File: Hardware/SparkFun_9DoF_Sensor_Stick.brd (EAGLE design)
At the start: 34.3 x 10.2 mm, 32 parts, among them U1 ITG-32001:1, U2 ADXL345", U3 3.3V/150mA, U4 HMC5883LSMD

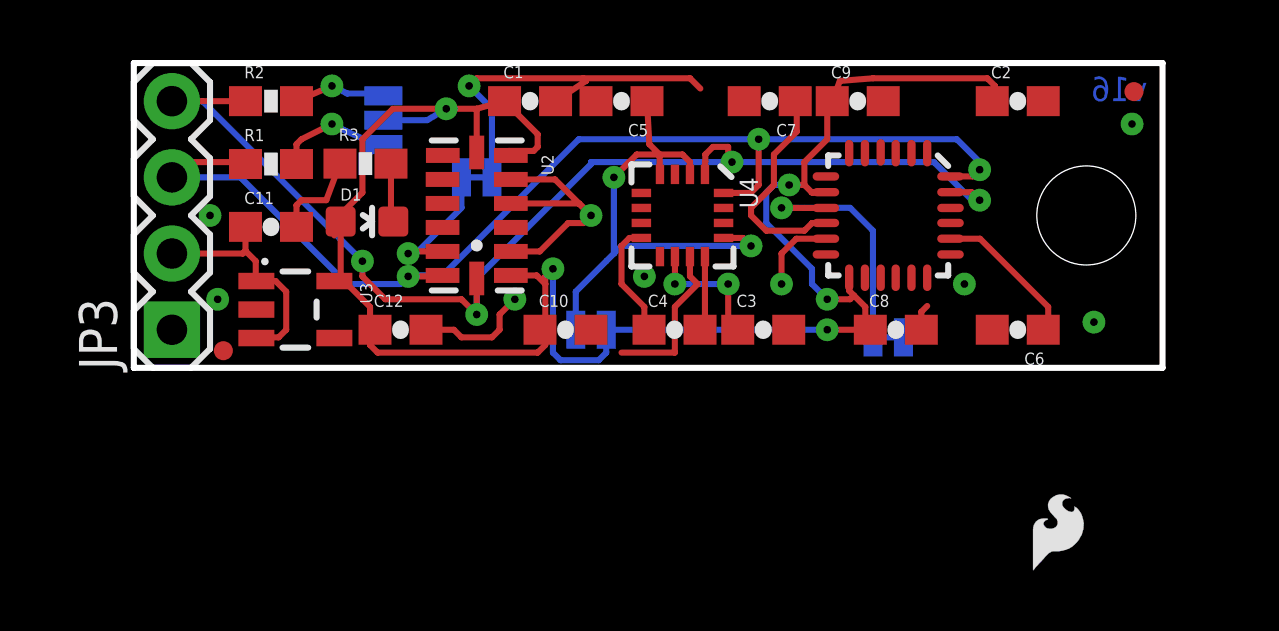
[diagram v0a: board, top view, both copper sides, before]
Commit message: BOARD PROTO LAYOUT
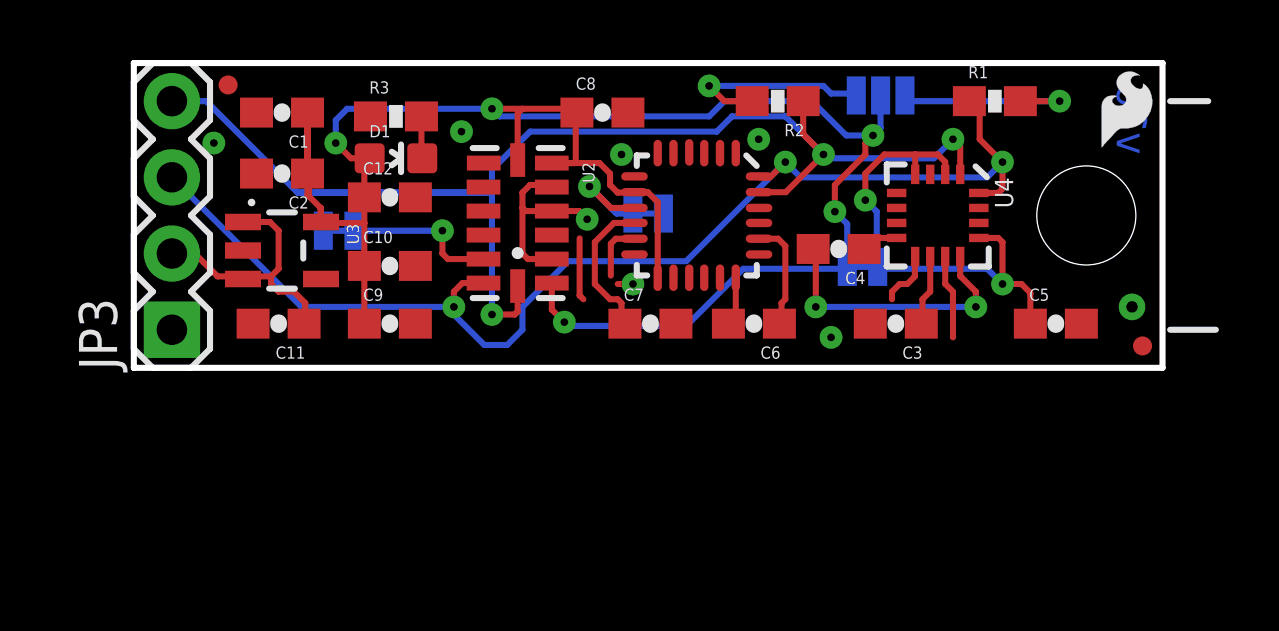
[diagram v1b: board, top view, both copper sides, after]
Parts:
- moved JP2 30.6 mm to (33.6, 0.73)
- moved JP1 30.2 mm to (3.14, 9.43)
- moved U$3 27.7 mm to (8.48, 1.75)
- moved C2 24.6 mm to (4.94, 6.48), turned to 180 degrees
- moved R1 24.2 mm to (28.7, 8.89)
- moved C9 17.3 mm to (8.53, 1.47)
- moved R2 16.9 mm to (21.5, 8.89), turned to 180 degrees
- moved SJ1 16.6 mm to (24.9, 9.08), turned to 180 degrees
- moved C5 16.3 mm to (30.7, 1.47), turned to 0 degrees
- moved JP4 14.3 mm to (31.9, 6.99)
- moved C8 12.2 mm to (15.6, 8.51)
- moved SJ4 9.29 mm to (24.3, 3.37), turned to 180 degrees
- moved SJ3 9.00 mm to (17.1, 5.14)
- moved C6 8.80 mm to (20.7, 1.47)
- moved U4 8.51 mm to (26.8, 5.08)
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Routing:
- net GND: track 37.8 -> 17.4 mm, vias 10 -> 8
- net SCL: track 40.8 -> 48.2 mm, vias 4 -> 3
- net N$3: track 2.51 -> 9.19 mm, vias 0 -> 2
- net N$9: track 8.40 -> 3.89 mm
- net N$8: track 3.09 -> 6.68 mm
- net N$2: track 3.95 -> 1.23 mm
- net N$6: track 3.95 -> 6.54 mm
- net 3.3V: track 65.2 -> 67.8 mm
- net N$7: track 7.28 -> 4.88 mm
- net N$1: track 4.44 -> 2.36 mm, vias 2 -> 0
- net SDA: track 38.8 -> 40.5 mm
- net N$5: track 5.03 -> 3.65 mm
- net N$12: track 17.3 -> 16.1 mm
- net VCC: track 7.97 -> 8.99 mm
- net N$4: track 2.30 -> 1.41 mm
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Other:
- board text added: "ACL"
- board text added: "ADD."
- board text added: "I2C"
- board text added: "MAG"
- board text added: "P/U"
